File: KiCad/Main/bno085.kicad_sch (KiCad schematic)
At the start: 24 parts, among them J10 RJ45, J2 Conn_01x02_Pin, J4 Conn_01x02_Pin, J7 RJ45, J9 RJ45, U1 ESP32-WROOM-32

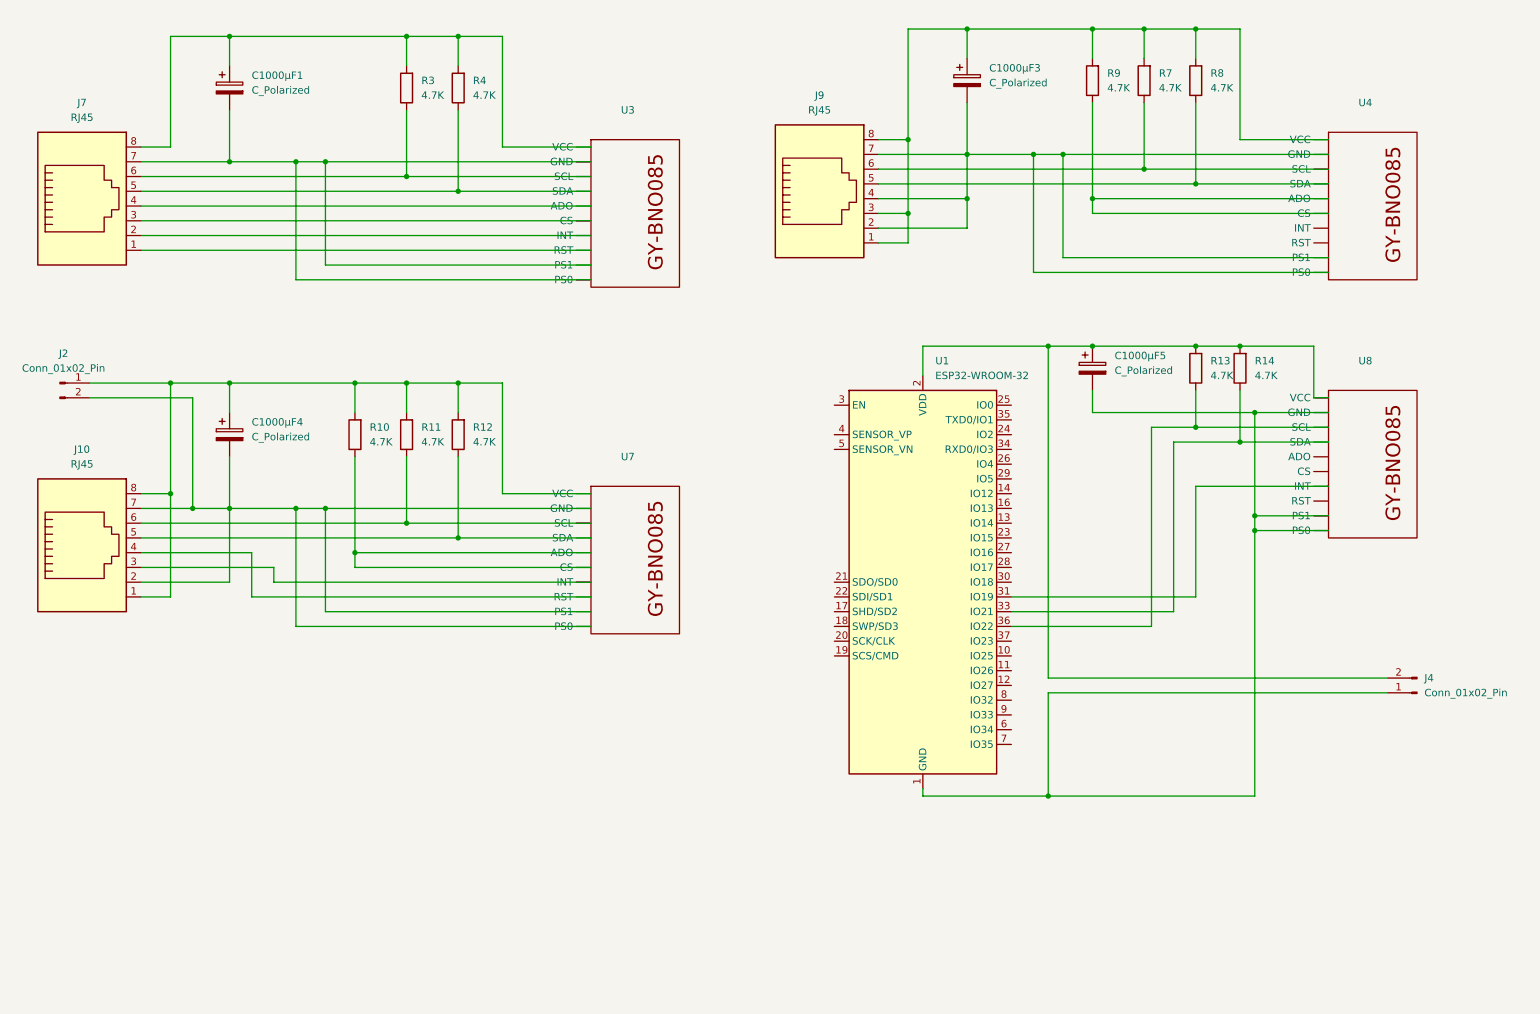
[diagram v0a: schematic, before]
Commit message: ok
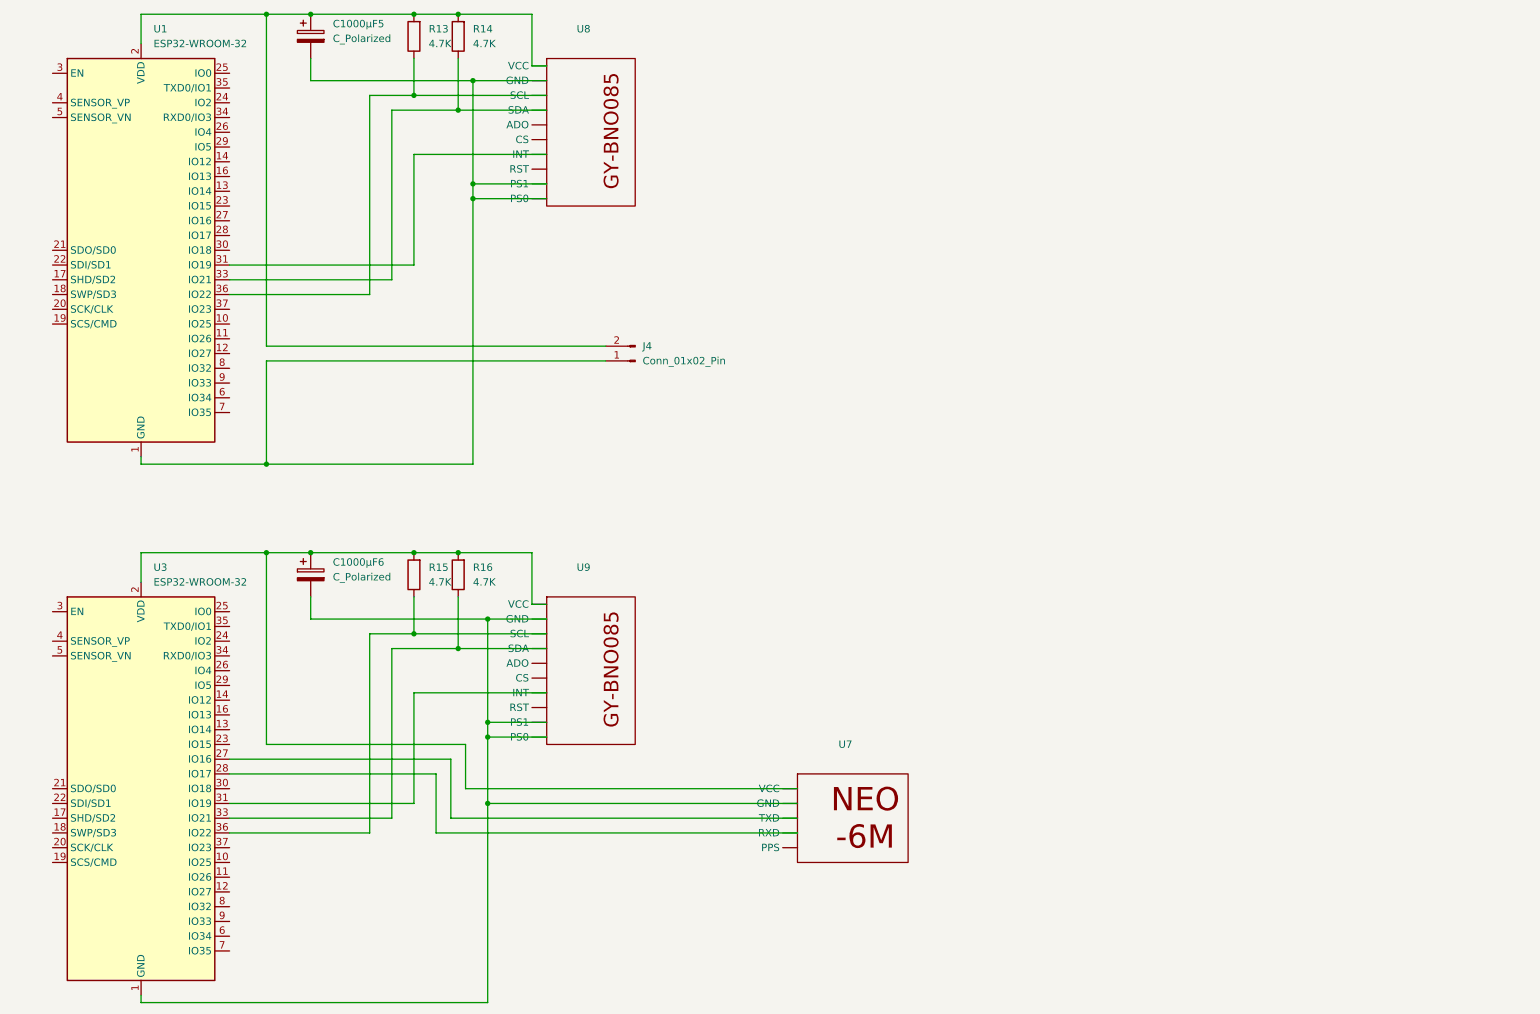
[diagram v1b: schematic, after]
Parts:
- removed C1000µF1, C1000µF3, C1000µF4: C_Polarized, Capacitor_THT:CP_Radial_D17.0mm_P7.50mm, symbol Device:C_Polarized
- removed J10, J7, J9: RJ45, Connector_RJ:RJ45_Amphenol_54602-x08_Horizontal, symbol Connector:RJ45
- removed J2: Conn_01x02_Pin, symbol Connector:Conn_01x02_Pin
- removed R10, R11, R12, R3, R4, R7, R8, R9: 4.7K, symbol Device:R
- removed U3, U4, U7: (no value), symbol gy-bno08x:gy-bno08x
- added C1000µF6: C_Polarized, Capacitor_THT:CP_Radial_D17.0mm_P7.50mm, symbol Device:C_Polarized
- added R15, R16: 4.7K, symbol Device:R
- added U3: ESP32-WROOM-32, RF_Module:ESP32-WROOM-32, symbol RF_Module:ESP32-WROOM-32
- added U7: (no value), symbol GH:NEO-6M
- added U9: (no value), symbol gy-bno08x:gy-bno08x
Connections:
- new net: R15.1, U3.36 (IO22), U9. (PS0)
- new net: C1000µF6.1, R15.2, R16.2, U3.2 (VDD), U7. (PPS), U9. (PS0)
- new net: R16.1, U3.33 (IO21), U9. (PS0)
- new net: C1000µF6.2, U3.1 (GND), U3.15 (GND), U3.38 (GND), U3.39 (GND), U7. (PPS), U9. (PS0)
- new net: U3.27 (IO16), U7. (PPS)
- new net: U3.28 (IO17), U7. (PPS)
- new net: U3.31 (IO19), U9. (PS0)
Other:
- moved on the sheet: C1000µF5, J4, R13, R14, U1, U8
